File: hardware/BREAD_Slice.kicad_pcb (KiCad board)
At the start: 2 copper layers, 72.6 x 100 mm, 16 parts, among them J1 Conn_01x10_Female, J2 I2C_01x04

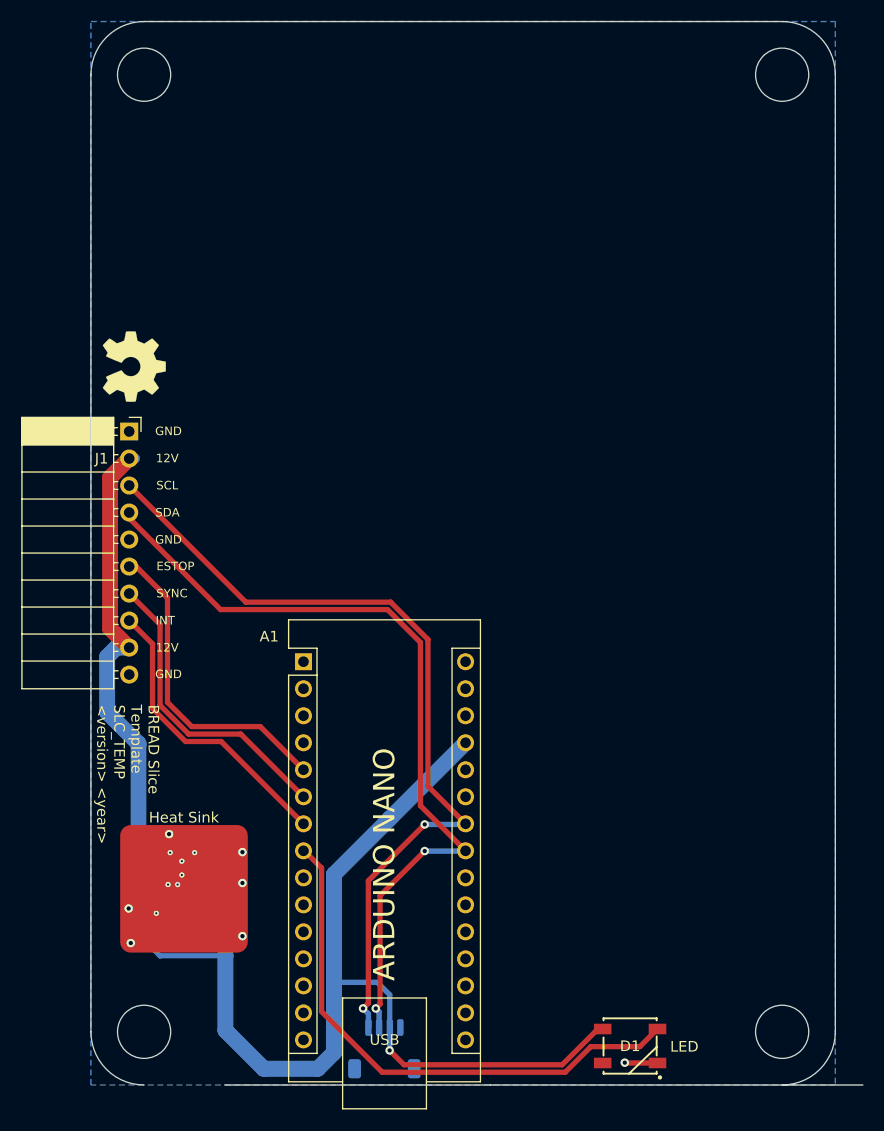
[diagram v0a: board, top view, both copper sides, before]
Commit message: Initial commit
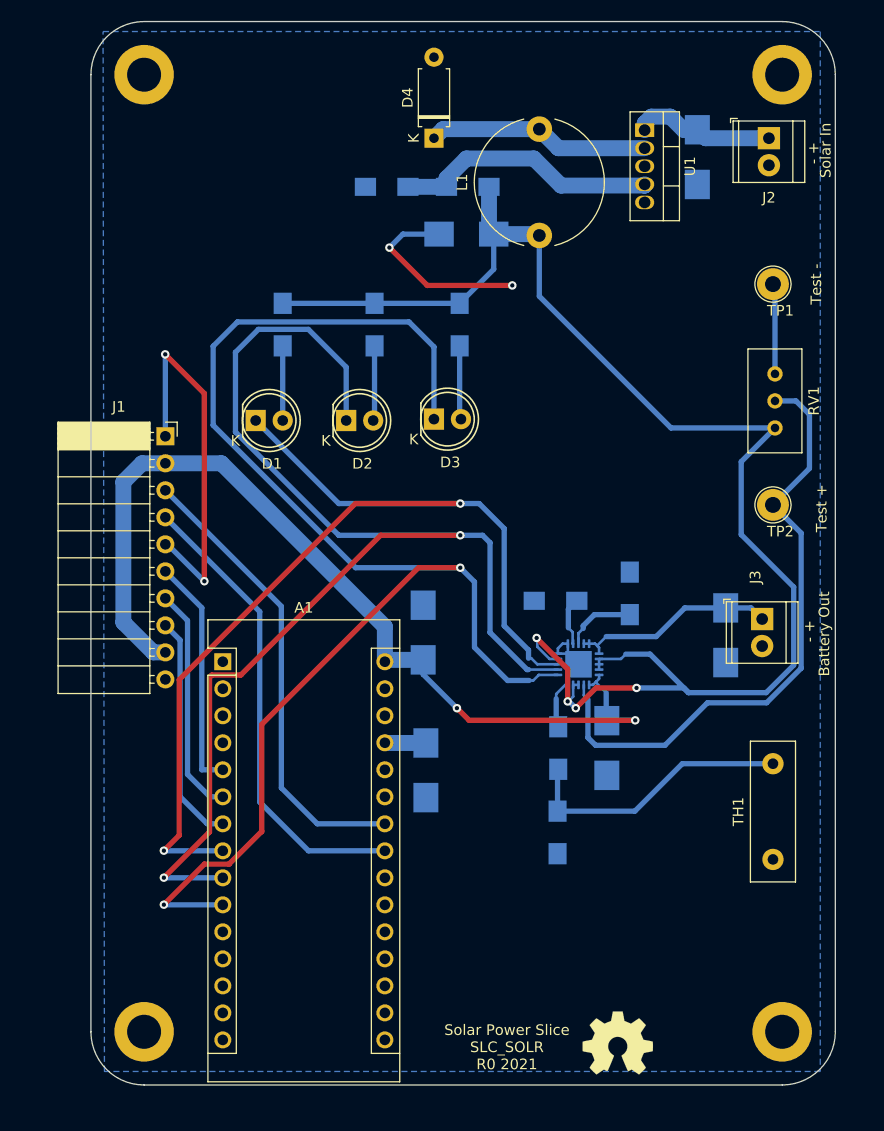
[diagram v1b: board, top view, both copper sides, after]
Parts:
- removed HS1: Heatsink_Pad, SparkFun-Fuse:Thermal Pad
- added C5: 10uF_t, OCI_UPL_FOOTPRINTS:C_2312, B.Cu at (171.1, 108.1)
- added C6: 10uF_t, OCI_UPL_FOOTPRINTS:C_2312, B.Cu at (182.3, 97.5)
- added D2: LED, OCI_UPL_FOOTPRINTS:LED-5MM, F.Cu at (146.6, 77.3)
- added D3: LED, OCI_UPL_FOOTPRINTS:LED-5MM, F.Cu at (154.9, 77.2)
- added D4: D_Schottky, Diode_THT:D_A-405_P7.62mm_Horizontal, F.Cu at (154.9, 50.8)
- added J3: Screw_Terminal_01x02, TerminalBlock_TE-Connectivity:TerminalBlock_TE_282834-2_1x02_P2.54mm_Horizontal, F.Cu at (185.7, 96.0)
- added R1: 1k, OCI_UPL_FOOTPRINTS:R_1206_HandSoldering, B.Cu at (140.6, 68.3)
- added R2: 1k, OCI_UPL_FOOTPRINTS:R_1206_HandSoldering, B.Cu at (149.3, 68.3)
- added R3: 1k, OCI_UPL_FOOTPRINTS:R_1206_HandSoldering, B.Cu at (157.3, 68.3)
- added R4: 5k, OCI_UPL_FOOTPRINTS:R_1206_HandSoldering, B.Cu at (158.0, 55.3)
- added R5: 1.2k, OCI_UPL_FOOTPRINTS:R_1206_HandSoldering, B.Cu at (150.4, 55.3)
- added R6: 100k, OCI_UPL_FOOTPRINTS:R_1206_HandSoldering, B.Cu at (166.5, 116.1)
- added R7: 2k, OCI_UPL_FOOTPRINTS:R_1206_HandSoldering, B.Cu at (173.3, 93.6)
- added R8: 100k, OCI_UPL_FOOTPRINTS:R_1206_HandSoldering, B.Cu at (166.3, 94.3)
- added R9: 1k, OCI_UPL_FOOTPRINTS:R_1206_HandSoldering, B.Cu at (166.5, 108.1)
- added RV1: 500k, Potentiometer_THT:Potentiometer_Bourns_3296W_Vertical, F.Cu at (186.9, 78.0)
- added TH1: 10k, Resistor_THT:R_Box_L13.0mm_W4.0mm_P9.00mm, F.Cu at (186.7, 118.6)
- added TP1: TestPoint, TestPoint:TestPoint_Loop_D2.54mm_Drill1.5mm_Beaded, F.Cu at (186.7, 64.5)
- added TP2: TestPoint, TestPoint:TestPoint_Loop_D2.54mm_Drill1.5mm_Beaded, F.Cu at (186.7, 85.3)
- added U2: MCP73871, Package_DFN_QFN:QFN-20-1EP_4x4mm_P0.5mm_EP2.5x2.5mm, B.Cu at (168.4, 100.2)
- C1: value 22uF -> 10uF_t; footprint Capacitor_SMD:C_1206_3216Metric -> OCI_UPL_FOOTPRINTS:C_2312
- C2: value 100nF -> 10uF_t; footprint Capacitor_SMD:C_1206_3216Metric -> OCI_UPL_FOOTPRINTS:C_2312
- C3: value 22uF -> 1000 uF; footprint Capacitor_SMD:C_1206_3216Metric -> OCI_UPL_FOOTPRINTS:C_2312
- C4: value 22uF -> 4700 uF; footprint Capacitor_SMD:C_1206_3216Metric -> OCI_UPL_FOOTPRINTS:C_2312
- D1: value WS2812B_5050 -> LED; footprint SparkFun-LED:WS2812-5050-4PIN -> OCI_UPL_FOOTPRINTS:LED-5MM
- H1, H4: footprint MountingHole:MountingHole_5mm -> MountingHole:MountingHole_3.2mm_M3_DIN965_Pad
- H2: renamed from H3; footprint MountingHole:MountingHole_5mm -> MountingHole:MountingHole_3.2mm_M3_DIN965_Pad
- H3: renamed from H2; footprint MountingHole:MountingHole_5mm -> MountingHole:MountingHole_3.2mm_M3_DIN965_Pad
- J2: value I2C_01x04 -> Screw_Terminal_01x02; footprint Connector_JST:JST_SH_SM04B-SRSS-TB_1x04-1MP_P1.00mm_Horizontal -> TerminalBlock_TE-Connectivity:TerminalBlock_TE_282834-2_1x02_P2.54mm_Horizontal; moved to F.Cu
- L1: value 4.7uH -> 100 uH; footprint Inductor_SMD:L_1210_3225Metric -> Inductor_THT:L_Radial_D12.0mm_P10.00mm_Neosid_SD12k_style1; moved to F.Cu
- U1: value ~ -> LM2576HVT-ADJ; footprint Package_TO_SOT_SMD:TSOT-23-6 -> Package_TO_SOT_THT:TO-220-5_Vertical; moved to F.Cu
- moved J2 92.9 mm to (186.4, 50.8), turned to -90 degrees
- moved U1 86.0 mm to (174.7, 50.0), turned to -90 degrees
- moved C4 78.6 mm to (179.6, 52.6), turned to -90 degrees
- moved Logo1 78.2 mm to (172.1, 135.9), turned to 0 degrees
- moved L1 70.0 mm to (164.8, 59.9), turned to 90 degrees
- moved D1 68.5 mm to (138.1, 77.3)
- moved C3 64.3 mm to (157.9, 59.8), turned to 180 degrees
- moved C1 33.7 mm to (153.8, 97.3), turned to 90 degrees
- moved C2 28.0 mm to (154.1, 110.2), turned to -90 degrees
- moved A1 7.59 mm to (135.0, 100.0)
- moved J1 3.43 mm to (129.6, 78.8)
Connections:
- A1 pad 1: unconnected-(A1-D1/TX-Pad1) -> Net-(A1-Pad1)
- A1 pad 10: unconnected-(A1-D7-Pad10) -> /PG
- A1 pad 11: unconnected-(A1-D8-Pad11) -> Net-(A1-Pad11)
- A1 pad 12: unconnected-(A1-D9-Pad12) -> Net-(A1-Pad12)
- A1 pad 13: unconnected-(A1-D10-Pad13) -> Net-(A1-Pad13)
- A1 pad 14: unconnected-(A1-D11-Pad14) -> Net-(A1-Pad14)
- A1 pad 15: unconnected-(A1-D12-Pad15) -> Net-(A1-Pad15)
- A1 pad 16: unconnected-(A1-D13-Pad16) -> Net-(A1-Pad16)
- A1 pad 17: unconnected-(A1-3V3-Pad17) -> Net-(A1-Pad17)
- A1 pad 18: unconnected-(A1-AREF-Pad18) -> Net-(A1-Pad18)
- A1 pad 19: unconnected-(A1-A0-Pad19) -> Net-(A1-Pad19)
- A1 pad 2: unconnected-(A1-D0/RX-Pad2) -> Net-(A1-Pad2)
- A1 pad 20: unconnected-(A1-A1-Pad20) -> Net-(A1-Pad20)
- A1 pad 21: unconnected-(A1-A2-Pad21) -> Net-(A1-Pad21)
- A1 pad 22: unconnected-(A1-A3-Pad22) -> Net-(A1-Pad22)
- A1 pad 25: unconnected-(A1-A6-Pad25) -> Net-(A1-Pad25)
- A1 pad 26: unconnected-(A1-A7-Pad26) -> Net-(A1-Pad26)
- A1 pad 28: unconnected-(A1-~{RESET}-Pad28) -> Net-(A1-Pad28)
- A1 pad 3: unconnected-(A1-~{RESET}-Pad3) -> Net-(A1-Pad3)
- A1 pad 30: unconnected-(A1-VIN-Pad30) -> /PWR
- A1 pad 8: /LED -> /CHG
- A1 pad 9: unconnected-(A1-D6-Pad9) -> /DONE
- C1 pad 1: GND -> /PWR
- C1 pad 2: +12V -> GND
- C2 pad 1: Net-(U1-SW) -> +5V
- C2 pad 2: Net-(U1-BST) -> GND
- C3 pad 1: GND -> VCC
- C3 pad 2: +5V -> GND
- C4 pad 1: GND -> Net-(C4-Pad1)
- C4 pad 2: +5V -> GND
- D1 pad 1: +5V -> /CHG
- D1 pad 2: unconnected-(D1-DOUT-Pad2) -> Net-(D1-Pad2)
- J1 pad 2: +12V -> /PWR
- J1 pad 9: +12V -> /PWR
- J2 pad 1: GND -> Net-(C4-Pad1)
- J2 pad 2: +5V -> GND
- L1 pad 1: Net-(U1-SW) -> VCC
- L1 pad 2: +5V -> Net-(D4-Pad1)
- U1 pad 1: +5V -> Net-(C4-Pad1)
- U1 pad 2: +12V -> Net-(D4-Pad1)
- U1 pad 3: +12V -> GND
- U1 pad 4: GND -> Net-(R4-Pad1)
- U1 pad 5: Net-(U1-SW) -> GND
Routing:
- net VCC: track 0.00 -> 139.2 mm, vias 0 -> 4
- net /PG: track 0.00 -> 135.5 mm, vias 0 -> 2
- net /DONE: track 0.00 -> 125.1 mm, vias 0 -> 2
- net +5V: track 108.9 -> 3.86 mm, vias 1 -> 0
- net /CHG: track 0.00 -> 99.2 mm, vias 0 -> 2
- net /PWR: track 0.00 -> 88.4 mm, vias 0 -> 2
- net Net-(RV1-Pad2): track 0.00 -> 58.6 mm
- net /LED: track 51.5 -> 0.00 mm
- net GND: track 19.6 -> 67.3 mm, vias 14 -> 4
- net +12V: track 46.8 -> 0.00 mm
- net /I2C_CLK: track 78.5 -> 43.6 mm, vias 2 -> 0
- net /I2C_DAT: track 76.6 -> 44.1 mm, vias 2 -> 0
- net Net-(R6-Pad2): track 0.00 -> 26.1 mm
- net Net-(R4-Pad1): track 0.00 -> 25.0 mm
- net Net-(D4-Pad1): track 0.00 -> 20.9 mm
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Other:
- board size 72.6 x 100 mm -> 70 x 100 mm
- board text added: "- +"
- board text added: "Battery Out"
- board text added: "Solar In"
- board text added: "Solar Power Slice SLC_SOLR R0 2021"
- board text added: "Test +"
- board text added: "Test -"
- board text removed: "12V"
- board text removed: "12V->5V Reg"
- board text removed: "5V I2C Connector"
- board text removed: "ARDUINO NANO"
- board text removed: "BREAD Slice Template SLC_TEMP <version> <year>"
- board text removed: "ESTOP"
- board text removed: "GND"
- board text removed: "INT"
- board text removed: "LED"
- board text removed: "SCL"
- board text removed: "SDA"
- board text removed: "SYNC"

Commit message: finished board
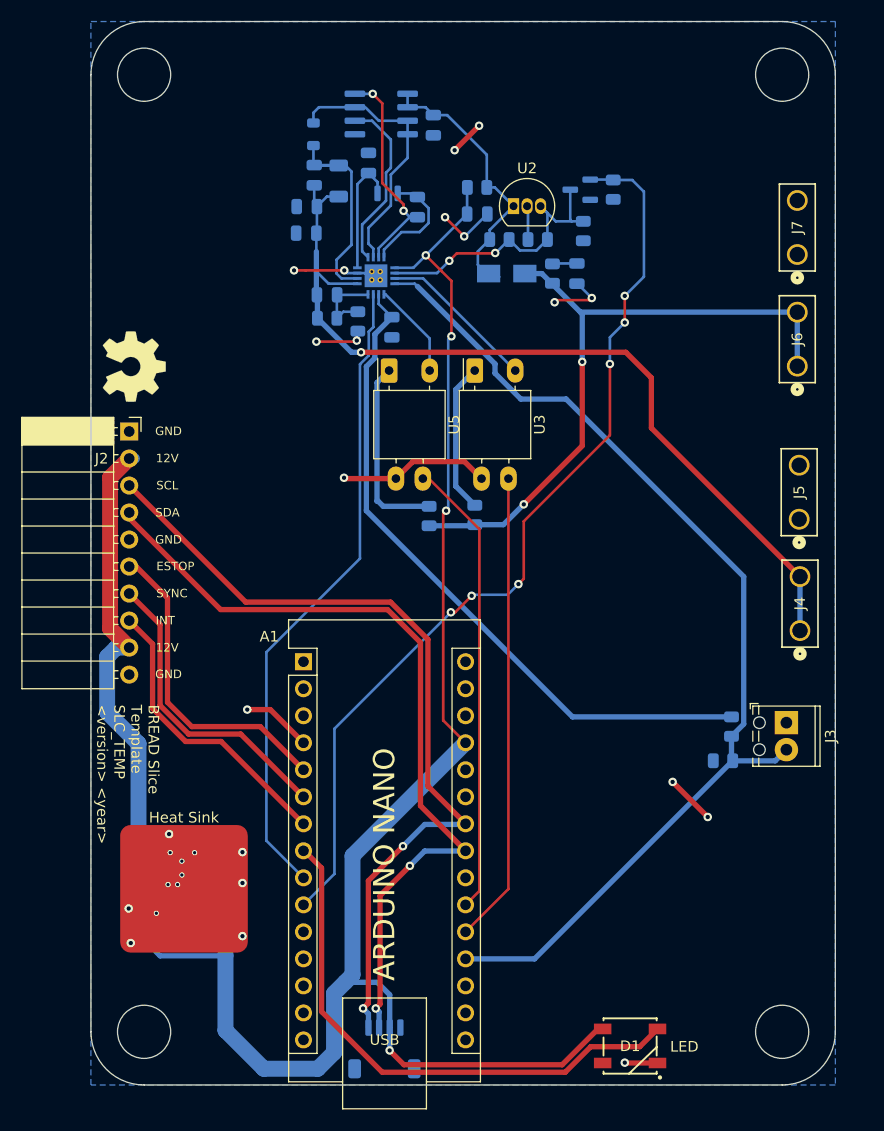
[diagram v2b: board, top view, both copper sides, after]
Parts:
- removed D4: D_Schottky, Diode_THT:D_A-405_P7.62mm_Horizontal
- removed the J2 at (186.4, 50.8)
- removed RV1: 500k, Potentiometer_THT:Potentiometer_Bourns_3296W_Vertical
- removed TH1: 10k, Resistor_THT:R_Box_L13.0mm_W4.0mm_P9.00mm
- removed TP1, TP2: TestPoint, TestPoint:TestPoint_Loop_D2.54mm_Drill1.5mm_Beaded
- added C10: 2.2uF, Capacitor_SMD:C_0805_2012Metric, B.Cu at (142.8, 59.7)
- added C11: 0.47u, Capacitor_SMD:C_0805_2012Metric, B.Cu at (158.9, 57.9)
- added C12: 4.7uF, Capacitor_SMD:C_0805_2012Metric, B.Cu at (142.9, 57.2)
- added C13: 22pF, Capacitor_SMD:C_0805_2012Metric, B.Cu at (144.8, 65.5)
- added C14: 1uF, Capacitor_SMD:C_0805_2012Metric, B.Cu at (150.9, 68.5)
- added C7: 1uF, Capacitor_SMD:C_0805_2012Metric, B.Cu at (148.7, 53.1)
- added C8: 0.1uF, Capacitor_SMD:C_0805_2012Metric, B.Cu at (143.6, 54.2)
- added C9: 10uF, Capacitor_SMD:C_0805_2012Metric, B.Cu at (154.8, 49.5)
- added HS1: Heatsink_Pad, SparkFun-Fuse:Thermal Pad, F.Cu at (131.3, 121.4)
- added J1: I2C_01x04, Connector_JST:JST_SH_SM04B-SRSS-TB_1x04-1MP_P1.00mm_Horizontal, B.Cu at (150.2, 136.4)
- added J4: Tab_Amp_1217861-1, KML-Custom:CONN_1217861-1_TEC, F.Cu at (189.3, 97.1)
- added J5: Tab_Amp_1217861-1, KML-Custom:CONN_1217861-1_TEC, F.Cu at (189.2, 86.6)
- added J6: Tab_Amp_1217861-1, KML-Custom:CONN_1217861-1_TEC, F.Cu at (189.0, 72.2)
- added J7: Tab_Amp_1217861-1, KML-Custom:CONN_1217861-1_TEC, F.Cu at (189.0, 61.7)
- added L2: 22uH, Inductor_SMD:L_0805_2012Metric, B.Cu at (143.5, 50.4)
- added Q1: AO4882, Package_SO:SOIC-8_3.9x4.9mm_P1.27mm, B.Cu at (149.9, 48.5)
- added Q2: 2N7002, Package_TO_SOT_SMD:SOT-23, B.Cu at (168.6, 55.6)
- added R10: 100k, Resistor_SMD:R_0805_2012Metric, B.Cu at (147.7, 68.0)
- added R11: 10k, Resistor_SMD:R_0805_2012Metric, B.Cu at (158.7, 86.2)
- added R12: 10k, Resistor_SMD:R_0805_2012Metric, B.Cu at (154.4, 86.3)
- added Rset1: 1k, Resistor_SMD:R_0805_2012Metric, B.Cu at (164.6, 60.3)
- added U3: NSL-32, OptoDevice:Luna_NSL-32, F.Cu at (158.7, 72.6)
- added U4: BQ24650RVAT, KML-Custom:RVA16_2P14X2P14, B.Cu at (149.4, 63.7)
- added U5: NSL-32, OptoDevice:Luna_NSL-32, F.Cu at (150.6, 72.6)
- C1: value 10uF_t -> 22uF; footprint OCI_UPL_FOOTPRINTS:C_2312 -> Capacitor_SMD:C_1206_3216Metric
- C2: value 10uF_t -> 100nF; footprint OCI_UPL_FOOTPRINTS:C_2312 -> Capacitor_SMD:C_1206_3216Metric
- C3: value 1000 uF -> 22uF; footprint OCI_UPL_FOOTPRINTS:C_2312 -> Capacitor_SMD:C_1206_3216Metric
- C4: value 4700 uF -> 22uF; footprint OCI_UPL_FOOTPRINTS:C_2312 -> Capacitor_SMD:C_1206_3216Metric
- C5: value 10uF_t -> 0.1uF; footprint OCI_UPL_FOOTPRINTS:C_2312 -> Capacitor_SMD:C_0805_2012Metric
- C6: value 10uF_t -> 2.2u; footprint OCI_UPL_FOOTPRINTS:C_2312 -> Capacitor_SMD:C_0805_2012Metric
- D1: value LED -> WS2812B_5050; footprint OCI_UPL_FOOTPRINTS:LED-5MM -> SparkFun-LED:WS2812-5050-4PIN
- D2: value LED -> BAT54C; footprint OCI_UPL_FOOTPRINTS:LED-5MM -> Package_TO_SOT_SMD:SOT-23; moved to B.Cu
- D3: value LED -> CDBA140-G; footprint OCI_UPL_FOOTPRINTS:LED-5MM -> KML-Custom:CDBA-G; moved to B.Cu
- H1, H4: footprint MountingHole:MountingHole_3.2mm_M3_DIN965_Pad -> MountingHole:MountingHole_5mm
- H2: renamed from H3; footprint MountingHole:MountingHole_3.2mm_M3_DIN965_Pad -> MountingHole:MountingHole_5mm
- H3: renamed from H2; footprint MountingHole:MountingHole_3.2mm_M3_DIN965_Pad -> MountingHole:MountingHole_5mm
- J3: value Screw_Terminal_01x02 -> Conn_01x02_Female; footprint TerminalBlock_TE-Connectivity:TerminalBlock_TE_282834-2_1x02_P2.54mm_Horizontal -> TerminalBlock_Phoenix:TerminalBlock_Phoenix_MPT-0,5-2-2.54_1x02_P2.54mm_Horizontal
- L1: value 100 uH -> 4.7uH; footprint Inductor_THT:L_Radial_D12.0mm_P10.00mm_Neosid_SD12k_style1 -> Inductor_SMD:L_1210_3225Metric; moved to B.Cu
- R1: value 1k -> 2; footprint OCI_UPL_FOOTPRINTS:R_1206_HandSoldering -> Resistor_SMD:R_0805_2012Metric
- R2: value 1k -> 10k; footprint OCI_UPL_FOOTPRINTS:R_1206_HandSoldering -> Resistor_SMD:R_0805_2012Metric
- R3: value 1k -> 5.23k; footprint OCI_UPL_FOOTPRINTS:R_1206_HandSoldering -> Resistor_SMD:R_0805_2012Metric
- R4: value 5k -> 30.1k; footprint OCI_UPL_FOOTPRINTS:R_1206_HandSoldering -> Resistor_SMD:R_0805_2012Metric
- R5: value 1.2k -> 169k; footprint OCI_UPL_FOOTPRINTS:R_1206_HandSoldering -> Resistor_SMD:R_0805_2012Metric
- R6: value 100k -> 10.6k; footprint OCI_UPL_FOOTPRINTS:R_1206_HandSoldering -> Resistor_SMD:R_0805_2012Metric
- R7: value 2k -> 80m - sense res; footprint OCI_UPL_FOOTPRINTS:R_1206_HandSoldering -> Resistor_SMD:R_1206_3216Metric
- R8: value 100k -> 20; footprint OCI_UPL_FOOTPRINTS:R_1206_HandSoldering -> Resistor_SMD:R_0805_2012Metric
- R9: value 1k -> 300k; footprint OCI_UPL_FOOTPRINTS:R_1206_HandSoldering -> Resistor_SMD:R_0805_2012Metric
- U1: value LM2576HVT-ADJ -> ~; footprint Package_TO_SOT_THT:TO-220-5_Vertical -> Package_TO_SOT_SMD:TSOT-23-6; moved to B.Cu
- U2: value MCP73871 -> LM234Z-3; footprint Package_DFN_QFN:QFN-20-1EP_4x4mm_P0.5mm_EP2.5x2.5mm -> Package_TO_SOT_THT:TO-92_Inline; moved to F.Cu
- moved U1 86.0 mm to (128.8, 122.8), turned to 0 degrees
- moved C4 78.6 mm to (133.8, 116.5), turned to 0 degrees
- moved Logo1 78.2 mm to (126.7, 72.2), turned to -90 degrees
- moved L1 70.0 mm to (133.8, 122.8), turned to 0 degrees
- moved D1 68.5 mm to (173.3, 136.1)
- moved C3 64.3 mm to (133.8, 119.5), turned to 0 degrees
- moved R4 59.1 mm to (182.0, 109.3), turned to 180 degrees
- moved R6 56.6 mm to (168.9, 59.5), turned to -90 degrees
- moved C5 53.9 mm to (153.3, 57.2)
- moved R7 47.5 mm to (145.9, 54.8), turned to -90 degrees
- moved R9 45.9 mm to (144.8, 67.7), turned to 180 degrees
- moved R3 45.6 mm to (182.8, 106.1), turned to -90 degrees
- moved U2 43.5 mm to (162.3, 57.2), turned to 0 degrees
- moved R8 39.6 mm to (158.9, 55.4)
- moved C6 36.8 mm to (168.3, 63.5)
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- renumbered J1 to J2
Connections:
- A1 pad 1: Net-(A1-Pad1) -> unconnected-(A1-D1/TX-Pad1)
- A1 pad 10: /PG -> /CHRG_EN
- A1 pad 11: Net-(A1-Pad11) -> unconnected-(A1-D8-Pad11)
- A1 pad 12: Net-(A1-Pad12) -> unconnected-(A1-D9-Pad12)
- A1 pad 13: Net-(A1-Pad13) -> unconnected-(A1-D10-Pad13)
- A1 pad 14: Net-(A1-Pad14) -> unconnected-(A1-D11-Pad14)
- A1 pad 15: Net-(A1-Pad15) -> unconnected-(A1-D12-Pad15)
- A1 pad 16: Net-(A1-Pad16) -> unconnected-(A1-D13-Pad16)
- A1 pad 17: Net-(A1-Pad17) -> unconnected-(A1-3V3-Pad17)
- A1 pad 18: Net-(A1-Pad18) -> unconnected-(A1-AREF-Pad18)
- A1 pad 19: Net-(A1-Pad19) -> /BAT_RTD
- A1 pad 2: Net-(A1-Pad2) -> unconnected-(A1-D0/RX-Pad2)
- A1 pad 20: Net-(A1-Pad20) -> /STAT1_IN
- A1 pad 21: Net-(A1-Pad21) -> /STAT2_IN
- A1 pad 22: Net-(A1-Pad22) -> unconnected-(A1-A3-Pad22)
- A1 pad 25: Net-(A1-Pad25) -> unconnected-(A1-A6-Pad25)
- A1 pad 26: Net-(A1-Pad26) -> unconnected-(A1-A7-Pad26)
- A1 pad 28: Net-(A1-Pad28) -> unconnected-(A1-~{RESET}-Pad28)
- A1 pad 3: Net-(A1-Pad3) -> unconnected-(A1-~{RESET}-Pad3)
- A1 pad 30: /PWR -> unconnected-(A1-VIN-Pad30)
- A1 pad 8: /CHG -> /LED
- A1 pad 9: /DONE -> /TERM_EN
- C1 pad 1: /PWR -> GND
- C1 pad 2: GND -> +12V
- C2 pad 1: +5V -> Net-(U1-SW)
- C2 pad 2: GND -> Net-(U1-BST)
- C3 pad 1: VCC -> GND
- C3 pad 2: GND -> +5V
- C4 pad 1: Net-(C4-Pad1) -> GND
- C4 pad 2: GND -> +5V
- C5 pad 1: /PWR -> /BQ24650 Solar Charger/BTST
- C5 pad 2: GND -> /BQ24650 Solar Charger/HIDRV
- D1 pad 1: /CHG -> +5V
- D1 pad 2: Net-(D1-Pad2) -> unconnected-(D1-DOUT-Pad2)
- D2 pad 1: /DONE -> /BQ24650 Solar Charger/REGN
- D2 pad 2: Net-(D2-Pad2) -> /BQ24650 Solar Charger/BTST
- D3 pad 1: /PG -> /BQ24650 Solar Charger/HIDRV_D
- D3 pad 2: Net-(D3-Pad2) -> /BQ24650 Solar Charger/SolarIn
- J2 pad 2: /PWR -> +12V
- J2 pad 9: /PWR -> +12V
- J3 pad 1: Net-(C6-Pad1) -> GND
- J3 pad 2: GND -> /BAT_RTD
- L1 pad 1: VCC -> Net-(U1-SW)
- L1 pad 2: Net-(D4-Pad1) -> +5V
- R1 pad 1: Net-(D1-Pad2) -> /BQ24650 Solar Charger/SolarIn
- R1 pad 2: VCC -> Net-(C6-Pad1)
- R2 pad 1: Net-(D2-Pad2) -> /CHRG_EN
- R2 pad 2: VCC -> GND
- R3 pad 1: Net-(D3-Pad2) -> /BQ24650 Solar Charger/VREF
- R3 pad 2: VCC -> /BAT_RTD
- R4 pad 1: Net-(R4-Pad1) -> /BAT_RTD
- R4 pad 2: VCC -> GND
- R5 pad 1: GND -> /BQ24650 Solar Charger/HIDRV_D
- R5 pad 2: Net-(R4-Pad1) -> /BQ24650 Solar Charger/MPPSET
- R6 pad 1: GND -> /BQ24650 Solar Charger/MPPSET
- R6 pad 2: Net-(R6-Pad2) -> GND
- R7 pad 1: Net-(R7-Pad1) -> /BQ24650 Solar Charger/SRP
- R7 pad 2: GND -> /BQ24650 Solar Charger/BatteryOut
- R8 pad 1: Net-(R8-Pad1) -> /BQ24650 Solar Charger/HIDRV_D
- R8 pad 2: GND -> +5V
- R9 pad 1: Net-(R9-Pad1) -> /BQ24650 Solar Charger/VFB
- R9 pad 2: Net-(R6-Pad2) -> /BQ24650 Solar Charger/BatteryOut
- U1 pad 1: Net-(C4-Pad1) -> +5V
- U1 pad 2: Net-(D4-Pad1) -> +12V
- U1 pad 3: GND -> +12V
- U1 pad 4: Net-(R4-Pad1) -> GND
- U1 pad 5: GND -> Net-(U1-SW)
- U2 pad 1: /PWR -> /BQ24650 Solar Charger/HIDRV_D
- U2 pad 3: VCC -> /BQ24650 Solar Charger/MPPSET
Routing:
- net +5V: track 3.86 -> 167.3 mm, vias 0 -> 4
- net VCC: track 139.2 -> 0.00 mm, vias 4 -> 0
- net /PG: track 135.5 -> 0.00 mm, vias 2 -> 0
- net /DONE: track 125.1 -> 0.00 mm, vias 2 -> 0
- net /BAT_RTD: track 0.00 -> 100.9 mm
- net /CHG: track 99.2 -> 0.00 mm, vias 2 -> 0
- net /PWR: track 88.4 -> 0.00 mm, vias 2 -> 0
- net /CHRG_EN: track 0.00 -> 88.0 mm, vias 0 -> 6
- net /BQ24650 Solar Charger/BatteryOut: track 0.00 -> 82.7 mm, vias 0 -> 1
- net /BQ24650 Solar Charger/VREF: track 0.00 -> 64.2 mm
- net /BQ24650 Solar Charger/SolarIn: track 0.00 -> 62.4 mm, vias 0 -> 2
- net /TERM_EN: track 0.00 -> 60.5 mm
- net Net-(Rset1-Pad1): track 58.6 -> 3.18 mm
- net /LED: track 0.00 -> 51.5 mm
- net +12V: track 0.00 -> 46.8 mm
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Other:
- outline, holes or cut-outs redrawn
- board text added: "12V"
- board text added: "12V->5V Reg"
- board text added: "5V I2C Connector"
- board text added: "ARDUINO NANO"
- board text added: "BREAD Slice Template SLC_TEMP <version> <year>"
- board text added: "ESTOP"
- board text added: "GND"
- board text added: "INT"
- board text added: "LED"
- board text added: "SCL"
- board text added: "SDA"
- board text added: "SYNC"
- board text removed: "- +"
- board text removed: "Battery Out"
- board text removed: "Solar In"
- board text removed: "Solar Power Slice SLC_SOLR R0 2021"
- board text removed: "Test +"
- board text removed: "Test -"
